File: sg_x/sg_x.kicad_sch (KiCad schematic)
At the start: 6 parts, among them IC1 TC118S, J1 Conn_01x03, J2 Conn_01x04, U1 ATtiny25-20SS

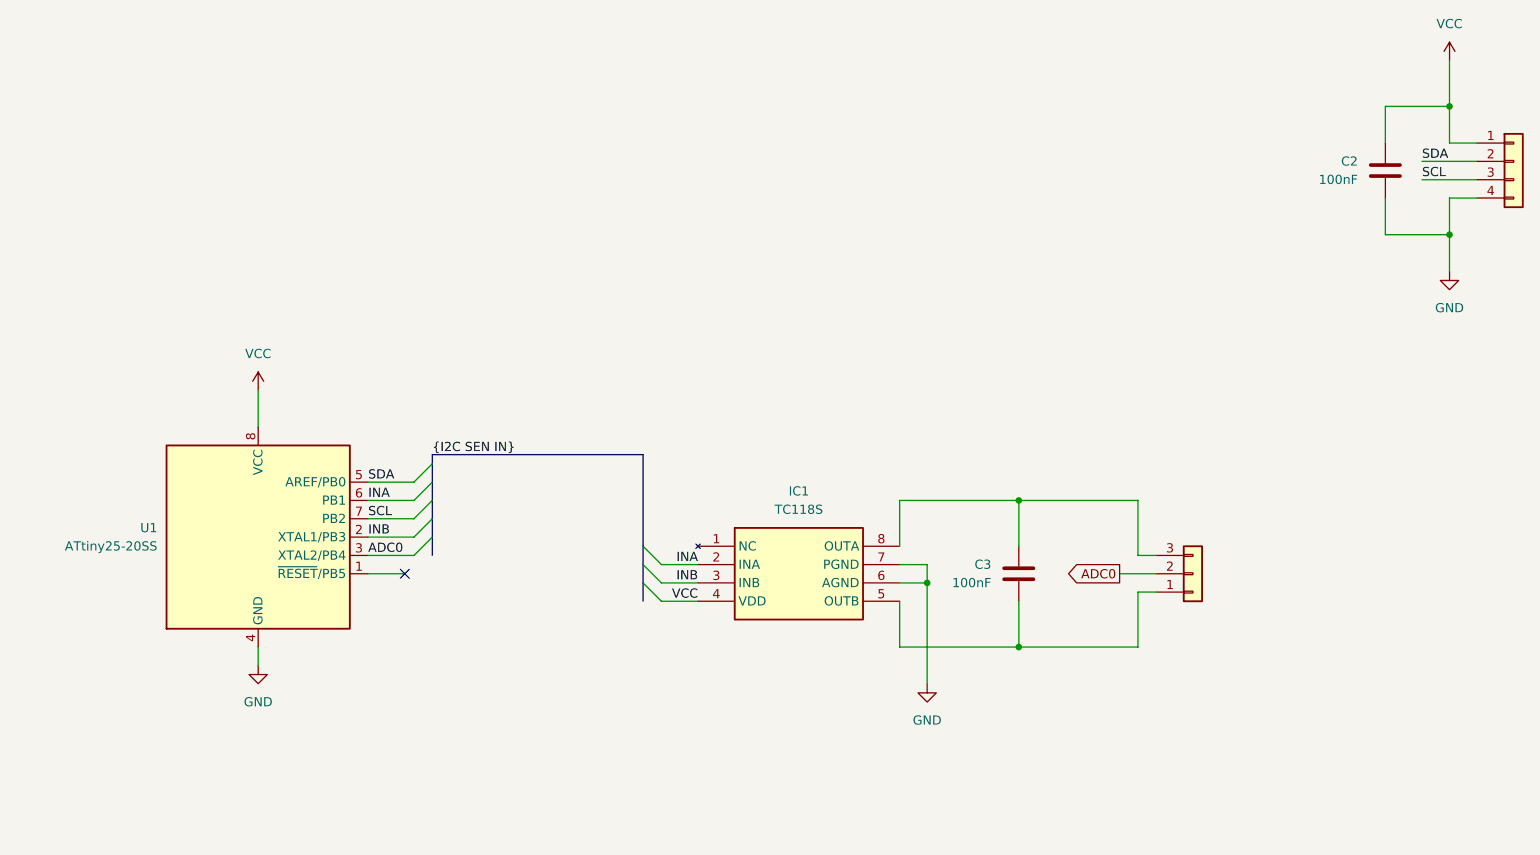
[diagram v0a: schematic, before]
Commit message: Minor changes
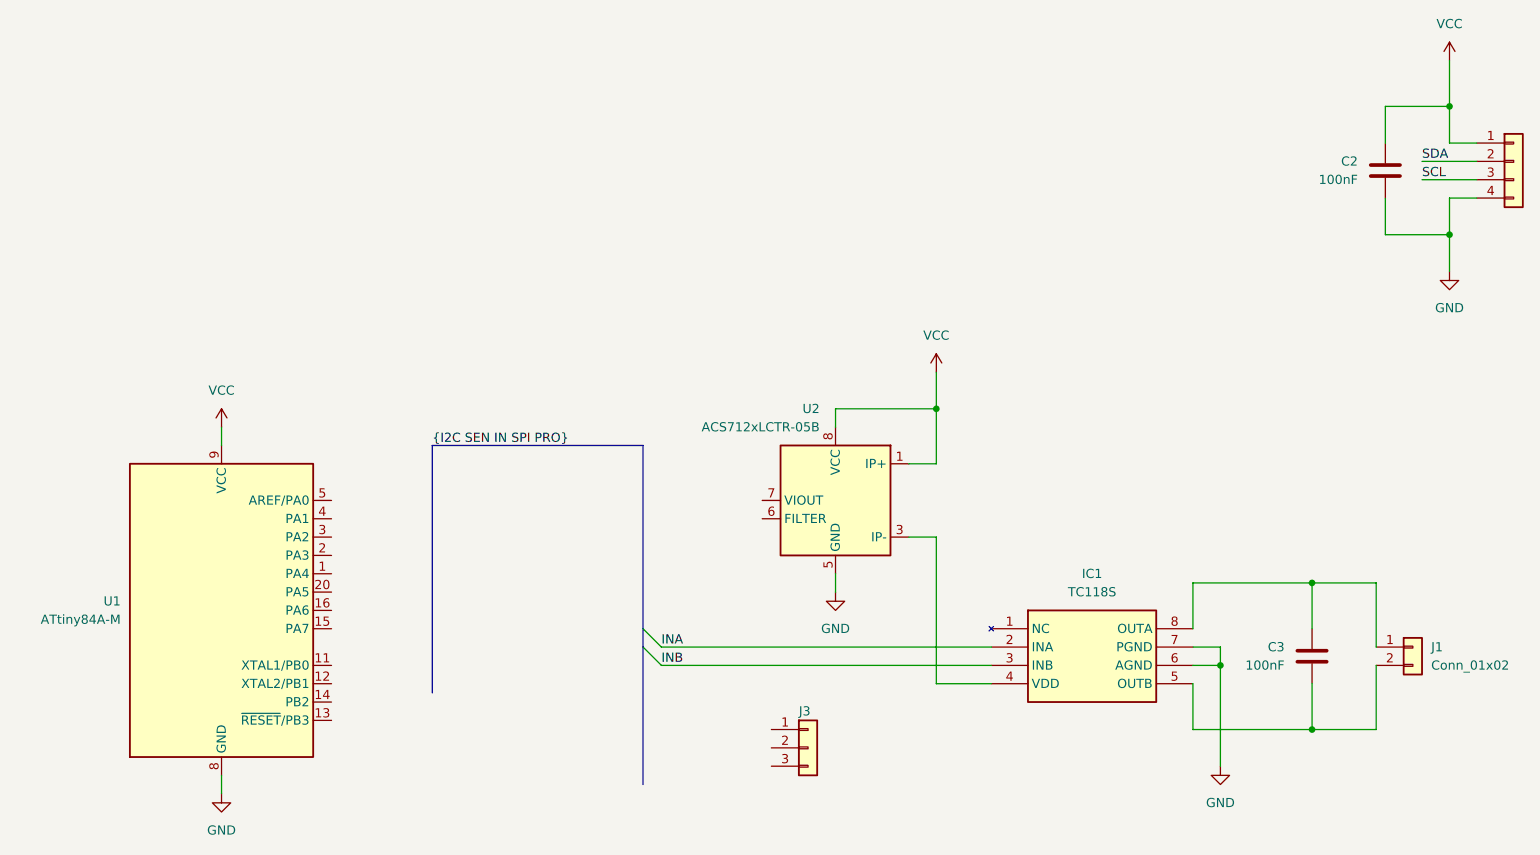
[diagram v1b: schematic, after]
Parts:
- removed J1: Conn_01x03, Connector_Servo_Driver:Connector_DC_Motor, symbol Connector_Generic:Conn_01x03
- removed U1: ATtiny25-20SS, Package_SO:SOIC-8_3.9x4.9mm_P1.27mm, symbol MCU_Microchip_ATtiny:ATtiny25-20SS
- added J1: Conn_01x02, Connector_Servo_Driver:Connector_DC_Motor, symbol Connector_Generic:Conn_01x02
- added J3: Conn_01x03, Connector_Servo_Driver:Connector_Servo_Driver_ADC, symbol Connector_Generic:Conn_01x03
- added U1: ATtiny84A-M, Package_DFN_QFN:QFN-20-1EP_4x4mm_P0.5mm_EP2.6x2.6mm, symbol MCU_Microchip_ATtiny:ATtiny84A-M
- added U2: ACS712xLCTR-05B, Package_SO:SOIC-8_3.9x4.9mm_P1.27mm, symbol Sensor_Current:ACS712xLCTR-05B
- IC1: footprint SOIC127P600X155-8N -> Package_SO:SOIC-8_3.9x4.9mm_P1.27mm
- J2: footprint Connector_Servo_Driver:Connector_Servo_Driver -> Connector_Servo_Driver:Connector_Servo_Driver_SMD
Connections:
- net GND: now also U1.21 (GND), U1.8 (GND), U2.5 (GND)
- net VCC: now also U1.9 (VCC), U2.1 (IP+), U2.2 (IP+), U2.8 (VCC); no longer IC1.4 (VDD)
- net at C3.1, IC1.8 (OUTA): now also J1.1 (Pin_1)
- net at C3.2, IC1.5 (OUTB): now also J1.2 (Pin_2)
- new net: IC1.4 (VDD), U2.3 (IP-), U2.4 (IP-)
- no-connect marks 1 -> 0
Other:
- moved on the sheet: C3, IC1
